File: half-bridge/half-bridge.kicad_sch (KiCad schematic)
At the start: 53 parts, among them J1 Conn_01x11_Pin, J2 Conn_01x11_Pin, J3 Conn_01x04_Pin, J4 Conn_01x04_Pin, J5 Conn_01x11_Pin, J6 Conn_01x11_Pin, J7 Conn_01x11_Pin, J8 Conn_01x11_Pin, Q1 GAN7R0-150LBE, Q2 GAN7R0-150LBE, U1 LMG1210

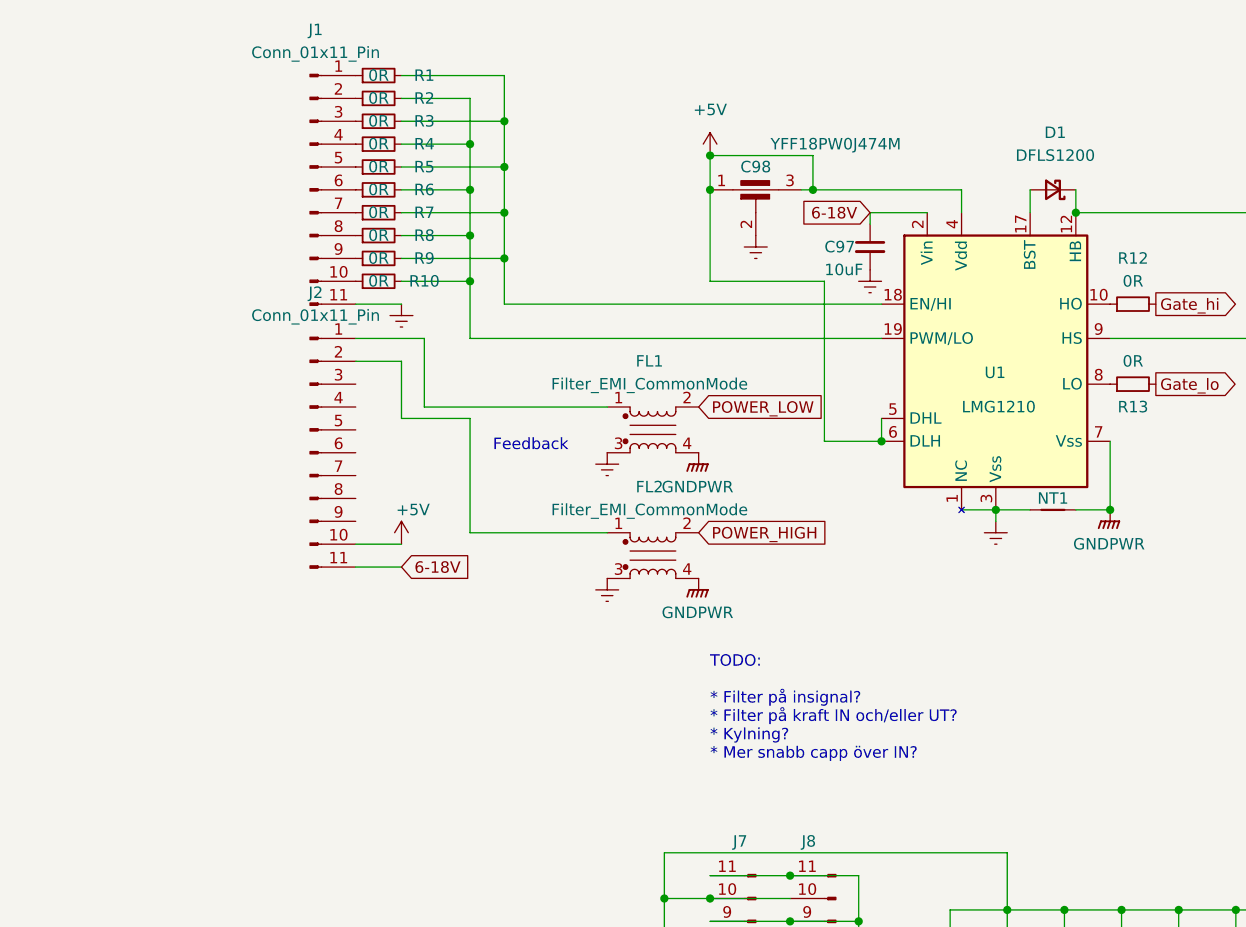
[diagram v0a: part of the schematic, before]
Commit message: Some changes
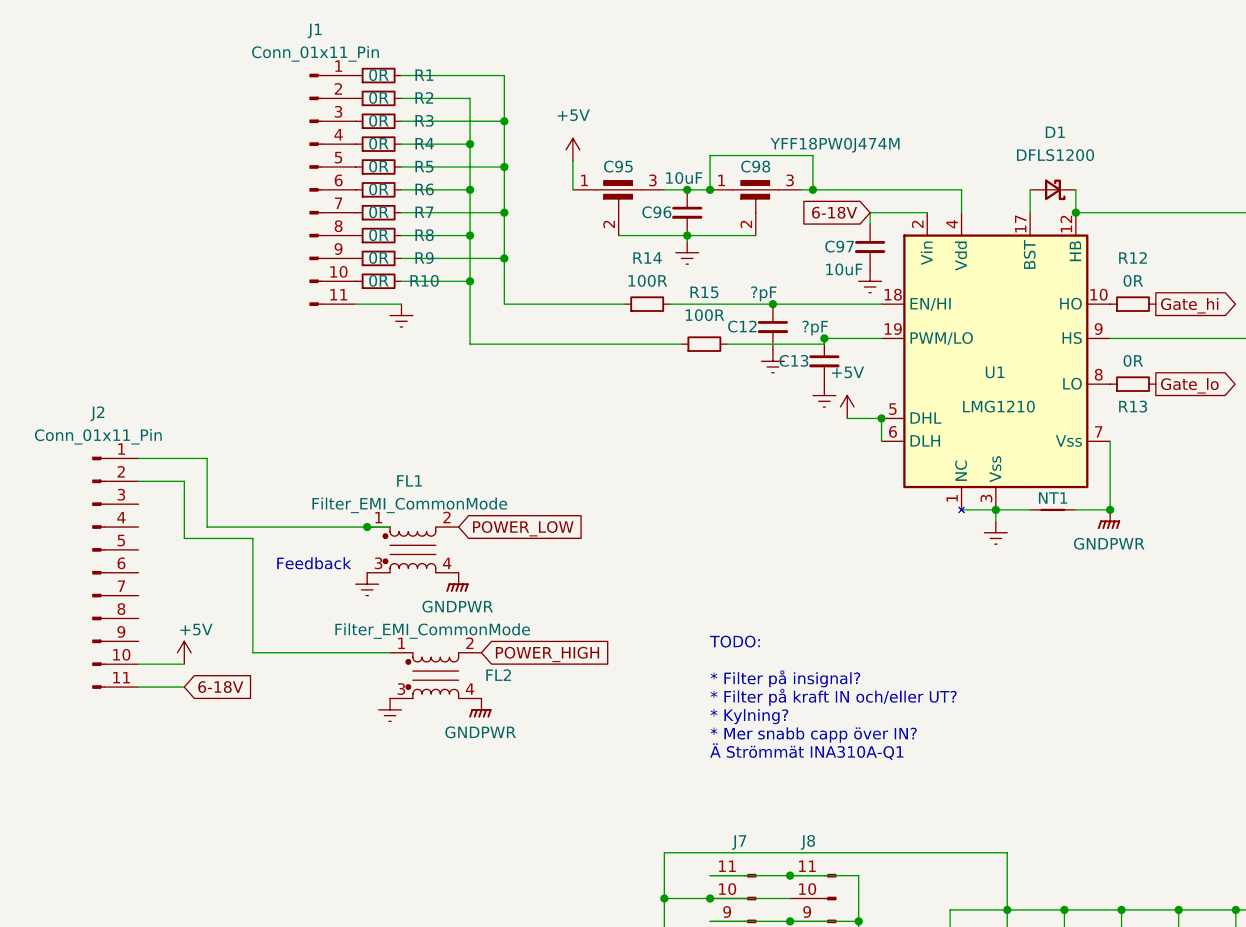
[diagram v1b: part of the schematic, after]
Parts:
- added C12, C13: ?pF, Capacitor_SMD:C_0402_1005Metric_Pad0.74x0.62mm_HandSolder, symbol Device:C_Small
- added C95: YFF18PW0J474M, Library:C_0603_1608Metric_Feedthrough_W_Vias, symbol Device:C_Feedthrough
- added C96: 10uF, Capacitor_SMD:C_0603_1608Metric, symbol Device:C_Small
- added R14, R15: 100R, Capacitor_SMD:C_0603_1608Metric, symbol Device:R_Small
- C98, C99: footprint Library:C_0603_1608Metric_Feedthrough -> Library:C_0603_1608Metric_Feedthrough_W_Vias
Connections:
- net +5V: now also C95.1; no longer C98.1, C98.3, U1.4 (Vdd)
- net Earth: now also C12.2, C13.2, C95.2, C96.2
- net at R10.2, R2.2, R4.2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: now also R15.1; no longer U1.19 (PWM/LO)
- net at R1.2, R3.2, R5.2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: now also R14.1; no longer U1.18 (EN/HI)
- new net: C13.1, R15.2, U1.19 (PWM/LO)
- new net: C12.1, R14.2, U1.18 (EN/HI)
- new net: C95.3, C96.1, C98.1, C98.3, U1.4 (Vdd)
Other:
- note added: "TODO: * Filter på insignal? * Filter på kraft IN och/eller UT? * Kylning? * Mer snabb capp över IN? Ä Strömmät INA310A-Q1"
- note removed: "TODO: * Filter på insignal? * Filter på kraft IN och/eller UT? * Kylning? * Mer snabb capp över IN?"
- moved on the sheet: FL1, FL2, J2
